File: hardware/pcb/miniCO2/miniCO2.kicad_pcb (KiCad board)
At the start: 4 copper layers, 17.3 x 17.7 mm, 12 parts, among them J1 USB_A, J2 Conn_01x04_Socket, SW1 SW_Push, U1 ATSAMD21E18A-M, U2 AP2112K-3.3, U3 SCD40-D-R2

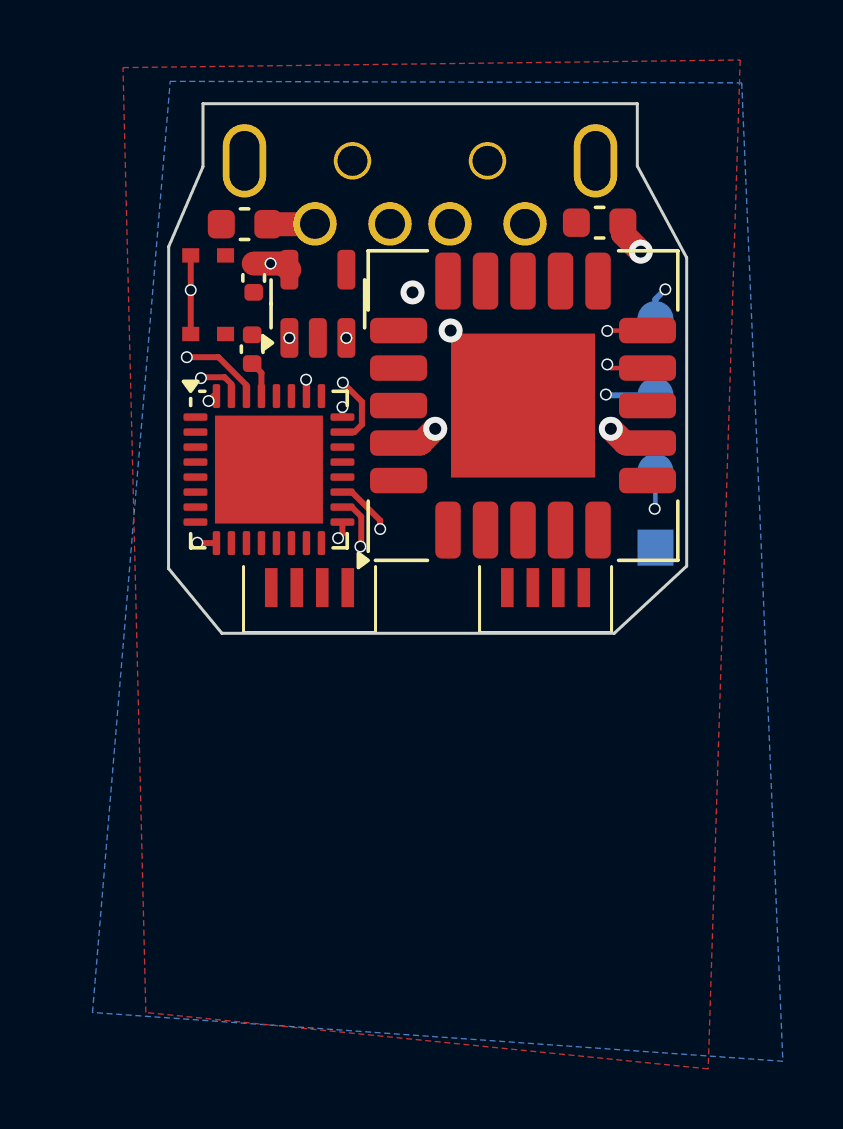
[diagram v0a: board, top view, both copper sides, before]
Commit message: Version 1 finished and sent to production
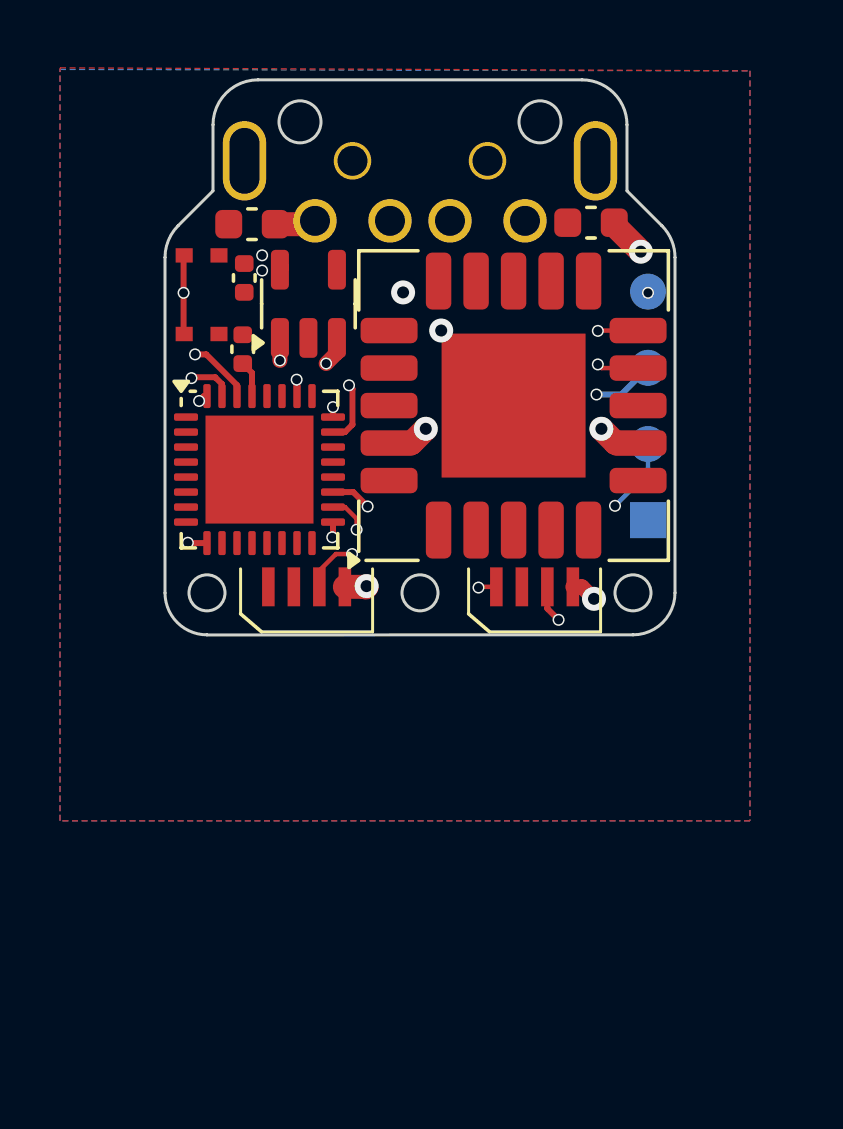
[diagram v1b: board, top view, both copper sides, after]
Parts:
- moved D2 7.97 mm to (137.6, 95.0)
- moved D1 7.50 mm to (145.2, 95.0)
- moved J2 0.95 mm to (149.0, 92.8)
- moved C3 0.31 mm to (135.6, 84.7)
- moved C4 0.31 mm to (135.5, 87.1)
- moved U1 0.31 mm to (136.1, 91.1)
- moved U2 0.31 mm to (137.7, 85.6)
- moved U3 0.31 mm to (144.5, 89.0)
- moved C2 0.29 mm to (147.1, 82.9)
- moved C1 0.25 mm to (135.8, 82.9)
- moved SW1 0.22 mm to (134.1, 85.3)
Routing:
- net DIN: track 1.93 -> 11.5 mm, vias 1 -> 2
- net Net-(D1-DOUT): track 0.00 -> 7.28 mm, vias 0 -> 2
- net VBUS: track 7.24 -> 9.44 mm
- net SWCLK: track 21.5 -> 20.1 mm
- net D+: track 7.90 -> 8.74 mm
- net SDA: track 13.8 -> 14.4 mm
- net +3.3V: track 8.86 -> 8.79 mm, vias 6 -> 9
- added copper zone on In1.Cu, net +3.3V
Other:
- board size 17.3 x 17.7 mm -> 17 x 18.5 mm
- board text added: "MINIC02"
- board text removed: "MINIC02 V1"
- board text removed: "MINICO2 V1"
